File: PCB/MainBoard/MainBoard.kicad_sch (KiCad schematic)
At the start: 54 parts, among them J1 Switch, J2 Prog Connector, J3 UART, J4 IR Connector, J5 R Motor, J6 L_Motor, J7 L_Motor_Backup, J8 R_Motor_Backup, J9 Backup connector bit, Q2 BSR802, SW1 RESET_SW, U1 MCP1700-3302E/TO, U2 ATmega4808-A

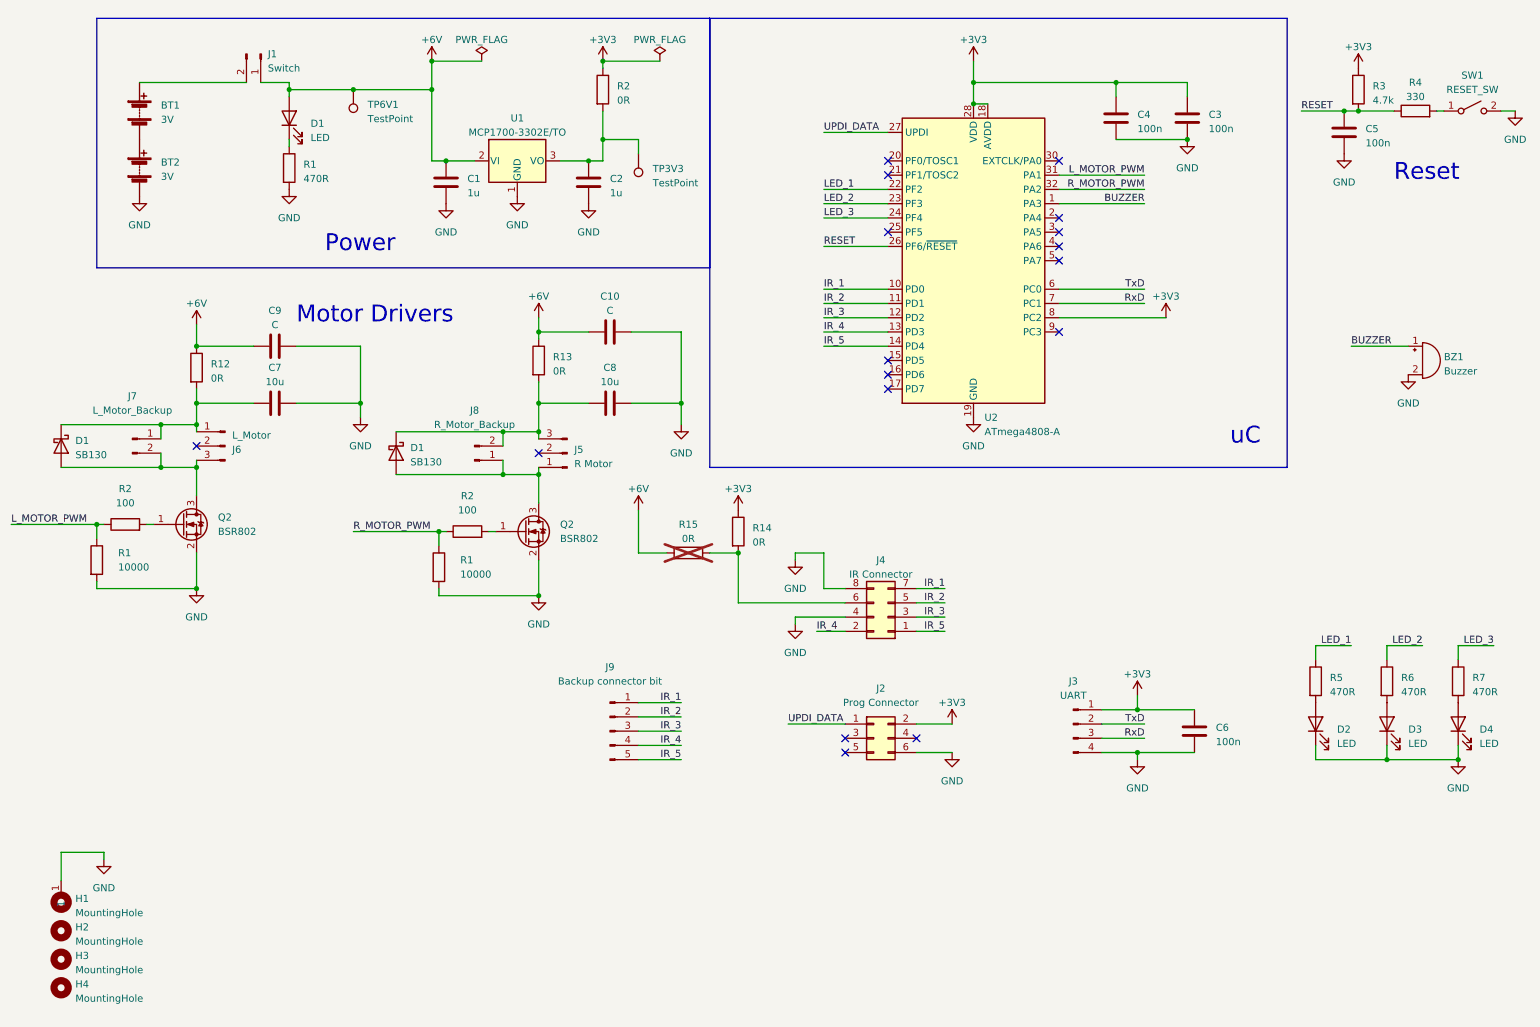
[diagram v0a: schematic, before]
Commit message: Cleaned up mainboard
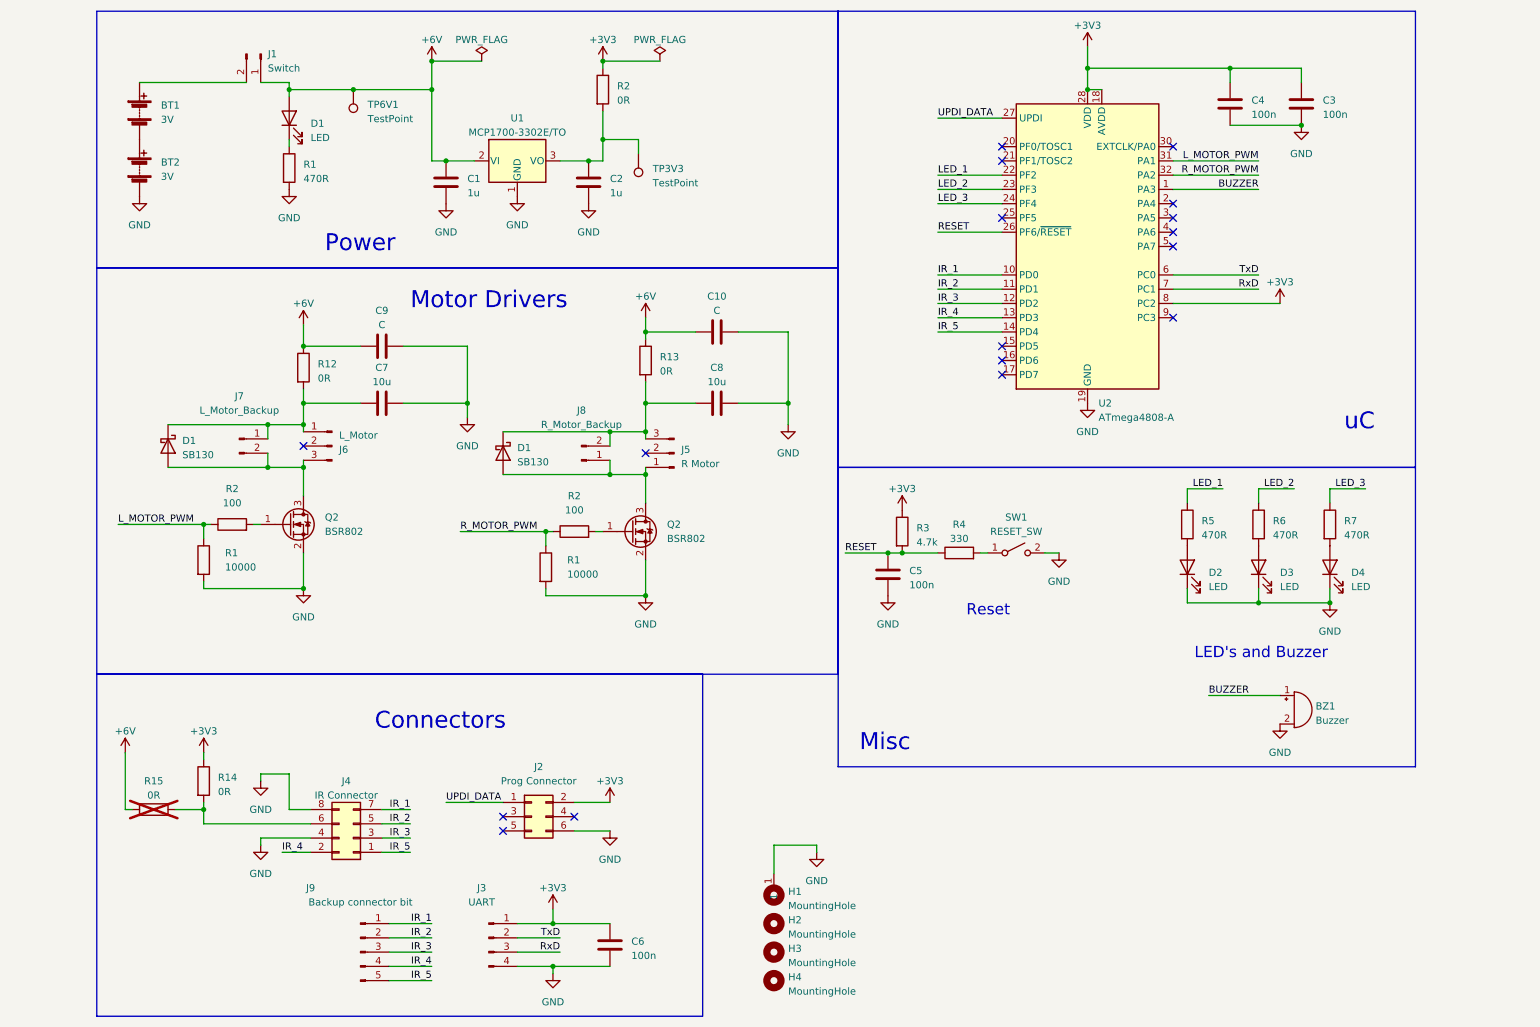
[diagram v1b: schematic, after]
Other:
- note added: "Connectors"
- note added: "LED's and Buzzer"
- note added: "Misc"
- moved on the sheet: BZ1, C10, C3, C4, C5, C6, C7, C8, C9, D1, D2, D3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
